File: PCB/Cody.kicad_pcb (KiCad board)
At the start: 2 copper layers, 87 x 114.5 mm, 30 parts, among them J1 Left Encoder, J12 12V Output, J13 Battery Discharge, J14 6V Input, J15 TCS34725 Color Sensor, J16 TCS34725 Color Sensor, J2 Right Encoder, J5 A1 Encoder, J6 A2 Encoder, J7 Battery Balance, J8 A3 Servo, J9 A4 Servo, U1 ESP32-DEVKITC-32D

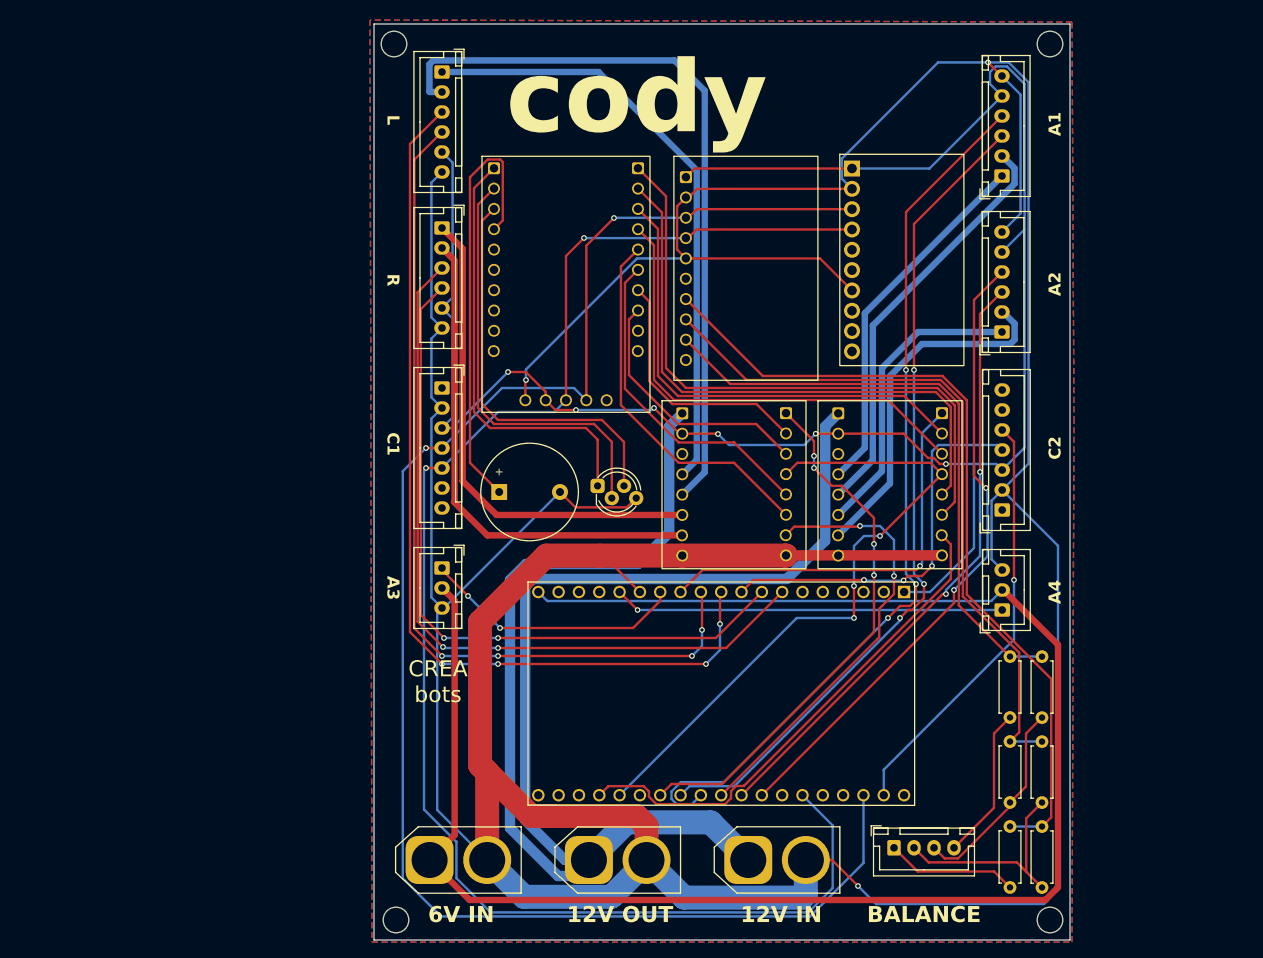
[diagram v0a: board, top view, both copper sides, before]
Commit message: 11-03-2026
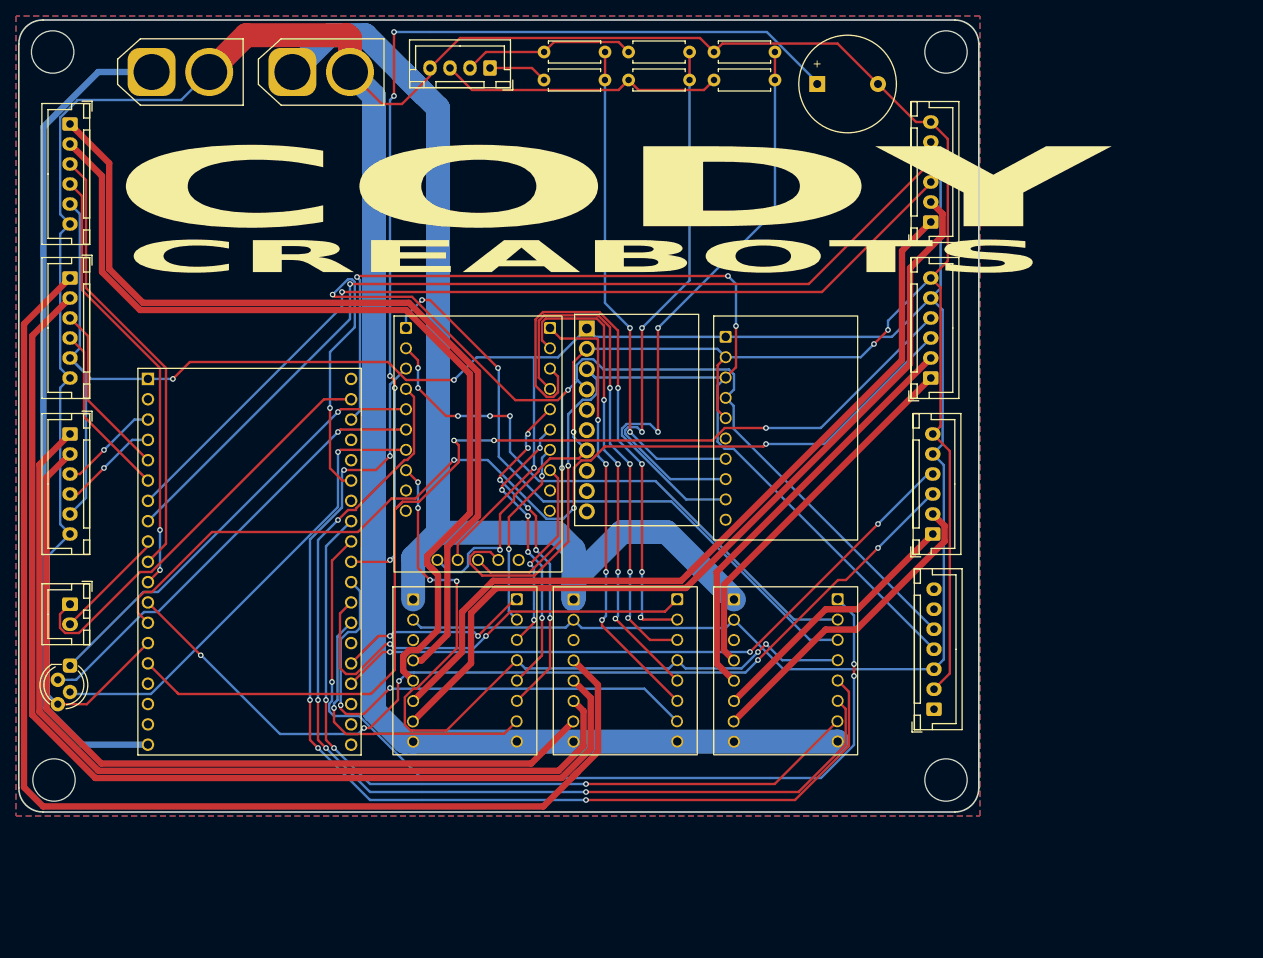
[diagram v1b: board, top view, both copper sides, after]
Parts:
- removed ? (x4): , 
- removed J12: 12V Output, Connector_AMASS:AMASS_XT60-F_1x02_P7.20mm_Vertical
- removed J16: TCS34725 Color Sensor, Connector_JST:JST_XH_B7B-XH-A_1x07_P2.50mm_Vertical
- removed J9: A4 Servo, Connector_JST:JST_XH_B3B-XH-A_1x03_P2.50mm_Vertical
- added J3: A3 Encoder, Connector_JST:JST_XH_B6B-XH-A_1x06_P2.50mm_Vertical, F.Cu at (146.6, 75.8)
- added J4: A4 Encoder, Connector_JST:JST_XH_B6B-XH-A_1x06_P2.50mm_Vertical, F.Cu at (146.8, 95.2)
- added REF**: MountingHole_5.3mm_M5, MountingHole:MountingHole_5.3mm_M5, F.Cu at (148.5, 35.0)
- added REF**: MountingHole_5.3mm_M5, MountingHole:MountingHole_5.3mm_M5, F.Cu at (36.8, 35.0)
- added REF**: MountingHole_5.3mm_M5, MountingHole:MountingHole_5.3mm_M5, F.Cu at (37.0, 126.0)
- added REF**: MountingHole_5.3mm_M5, MountingHole:MountingHole_5.3mm_M5, F.Cu at (148.5, 126.0)
- added U7: ~, Dependencies:TB6612FNG, F.Cu at (128.5, 111.3)
- J8: value A3 Servo -> Camera; footprint Connector_JST:JST_XH_B3B-XH-A_1x03_P2.50mm_Vertical -> Connector_JST:JST_XH_B2B-XH-A_1x02_P2.50mm_Vertical
- moved J5 117.2 mm to (39.0, 63.2), turned to -90 degrees
- moved J6 117.2 mm to (39.0, 82.8), turned to -90 degrees
- moved R1 116.5 mm to (98.2, 38.5), turned to 0 degrees
- moved J13 113.8 mm to (66.8, 37.5)
- moved R2 111.2 mm to (105.9, 35.0), turned to 180 degrees
- moved J7 109.8 mm to (91.5, 37.0), turned to 180 degrees
- moved R3 107.1 mm to (108.8, 35.0), turned to 0 degrees
- moved J14 104.5 mm to (49.2, 37.5)
- moved R4 91.9 mm to (116.4, 38.5), turned to 180 degrees
- moved R5 89.6 mm to (119.5, 38.5), turned to 0 degrees
- moved R6 81.1 mm to (127.1, 35.0), turned to 180 degrees
- moved J15 73.4 mm to (147.0, 117.2), turned to 90 degrees
- moved D1 69.7 mm to (39.0, 111.7), turned to -90 degrees
- moved U1 65.1 mm to (61.4, 95.6), turned to 0 degrees
- moved BZ1 64.7 mm to (132.4, 39.0)
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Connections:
- J7 pad 4: /BMS_IN_4 -> GND
- J8 pad 1: /A3 -> /CAM_TX
- J8 pad 2: +6V -> /CAM_RX
- R6 pad 2: /BMS_IN_4 -> GND
- U1 pad J2-12: /A1_PWM -> /A4_A
- U1 pad J2-13: /A3 -> /A3_A
- U1 pad J2-15: /A4 -> /A3_B
- U1 pad J2-3: unconnected-(U1-SENSOR_VP-PadJ2-3) -> /A2_A
- U1 pad J2-4: unconnected-(U1-SENSOR_VN-PadJ2-4) -> /A2_B
- U1 pad J2-5: unconnected-(U1-IO34-PadJ2-5) -> /A1_A
- U1 pad J2-6: unconnected-(U1-IO35-PadJ2-6) -> /A1_B
- U1 pad J2-9: /SCL_1 -> /CAM_RX
- U1 pad J3-10: /R_PWM -> /BUZZER
- U1 pad J3-11: /A1_B -> /A2_PWM
- U1 pad J3-12: /A1_A -> /A1_PWM
- U1 pad J3-13: /L_PWM -> /R_PWM
- U1 pad J3-15: /STNDBY -> /L_PWM
- U1 pad J3-16: /A2_PWM -> /A4_B
- U1 pad J3-2: /SDA_1 -> /CAM_TX
- U1 pad J3-8: /A2_B -> /A4_PWM
- U1 pad J3-9: /A2_A -> /A3_PWM
- U2 pad 3: (no net) -> unconnected-(U2-GND-Pad3)
- U3 pad 3: (no net) -> unconnected-(U3-GND-Pad3)
- U6 pad 1: /LED_R -> /A3_IN_1
- U6 pad 2: /LED_G -> /A3_IN_2
- U6 pad 3: /LED_B -> /A4_IN_1
- U6 pad 4: /BUZZER -> /A4_IN_2
- U6 pad 5: unconnected-(U6-P14-Pad5) -> /LED_R
- U6 pad 6: unconnected-(U6-P15-Pad6) -> /LED_G
- U6 pad 7: unconnected-(U6-P16-Pad7) -> /LED_B
- U6 pad 8: unconnected-(U6-P17-Pad8) -> /STNDBY
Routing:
- net /A4_IN_1: track 0.00 -> 135.8 mm, vias 0 -> 5
- net /A3_B: track 0.00 -> 134.2 mm, vias 0 -> 3
- net /A4_IN_2: track 0.00 -> 127.1 mm, vias 0 -> 4
- net /A3_A: track 0.00 -> 125.2 mm, vias 0 -> 3
- net /A4_A: track 0.00 -> 118.8 mm, vias 0 -> 5
- net +6V: track 216.8 -> 103.8 mm
- net /A3_PWM: track 0.00 -> 112.2 mm, vias 0 -> 3
- net /A1_OUT_1: track 45.8 -> 155.2 mm
- net /A4_PWM: track 0.00 -> 98.1 mm, vias 0 -> 3
- net /A1_B: track 111.8 -> 21.9 mm, vias 3 -> 0
- net /A1_OUT_2: track 52.1 -> 138.1 mm
- net /A4_B: track 0.00 -> 83.6 mm, vias 0 -> 3
- net /A1_A: track 103.7 -> 21.8 mm, vias 3 -> 0
- net /A3_IN_1: track 0.00 -> 80.3 mm, vias 0 -> 2
- net +3V3: track 244.6 -> 324.7 mm, vias 6 -> 3
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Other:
- board size 87 x 114.5 mm -> 120 x 99 mm
- board text added: "CODY"
- board text added: "CREABOTS"
- board text removed: "12V IN"
- board text removed: "12V OUT"
- board text removed: "6V IN"
- board text removed: "A1"
- board text removed: "A2"
- board text removed: "A3"
- board text removed: "A4"
- board text removed: "BALANCE"
- board text removed: "C1"
- board text removed: "C2"
- board text removed: "CREA bots"
- board text removed: "L"
- board text removed: "R"
- board text removed: "cody"

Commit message: 18-03-2026
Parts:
- added J10: Limit Switch 2, Connector_JST:JST_XH_B2B-XH-A_1x02_P2.50mm_Vertical, F.Cu at (100.0, 76.0)
- added J9: Limit Switch 1, Connector_JST:JST_XH_B2B-XH-A_1x02_P2.50mm_Vertical, F.Cu at (100.0, 85.2)
- added R7: R, Resistor_THT:R_Axial_DIN0207_L6.3mm_D2.5mm_P7.62mm_Horizontal, F.Cu at (121.0, 134.0)
- added SW3: SW_Push, Button_Switch_Keyboard:SW_Cherry_MX_1.00u_PCB, F.Cu at (99.4, 65.6)
- D1: value LED_RGBK -> LED; footprint LED_THT:LED_D5.0mm-4_RGB_Staggered_Pins -> LED_THT:LED_D3.0mm
- J8: footprint Connector_JST:JST_XH_B2B-XH-A_1x02_P2.50mm_Vertical -> Connector_JST:JST_XH_B4B-XH-A_1x04_P2.50mm_Vertical
- moved J14 166.7 mm to (208.5, 86.5), turned to -90 degrees
- moved J13 156.3 mm to (208.5, 103.5), turned to -90 degrees
- moved J8 148.5 mm to (175.5, 45.5), turned to 180 degrees
- moved J7 147.7 mm to (209.0, 126.5), turned to 90 degrees
- moved R2 140.4 mm to (203.4, 136.0)
- moved R1 135.5 mm to (195.8, 132.5)
- moved R3 123.8 mm to (185.2, 132.5)
- moved R4 123.8 mm to (192.8, 136.0)
- moved R5 112.1 mm to (174.8, 136.0)
- moved R6 112.1 mm to (182.4, 132.5)
- moved J6 107.2 mm to (139.5, 45.5), turned to 180 degrees
- moved J15 87.7 mm to (197.5, 45.5), turned to 180 degrees
- moved J5 82.4 mm to (119.5, 45.5), turned to 180 degrees
- moved U4 82.2 mm to (192.1, 90.3)
- moved J1 79.2 mm to (100.0, 94.5)
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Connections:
- D1 pad 1: /LED_R -> GND
- D1 pad 2: /LED_G -> Net-(D1-A)
- J1 pad 3: /L_A -> GND
- J1 pad 4: /L_B -> +3V3
- J1 pad 5: +3V3 -> /L_A
- J1 pad 6: GND -> /L_B
- J2 pad 3: /R_A -> GND
- J2 pad 4: /R_B -> +3V3
- J2 pad 5: +3V3 -> /R_A
- J2 pad 6: GND -> /R_B
- J3 pad 3: /A3_A -> GND
- J3 pad 4: /A3_B -> +3V3
- J3 pad 5: +3V3 -> /A3_A
- J3 pad 6: GND -> /A3_B
- J4 pad 3: /A4_A -> GND
- J4 pad 4: /A4_B -> +3V3
- J4 pad 5: +3V3 -> /A4_A
- J4 pad 6: GND -> /A4_B
- J5 pad 3: /A1_A -> GND
- J5 pad 4: /A1_B -> +3V3
- J5 pad 5: +3V3 -> /A1_A
- J5 pad 6: GND -> /A1_B
- J6 pad 3: /A2_A -> GND
- J6 pad 4: /A2_B -> +3V3
- J6 pad 5: +3V3 -> /A2_A
- J6 pad 6: GND -> /A2_B
- J8 pad 1: /CAM_TX -> +6V
- J8 pad 2: /CAM_RX -> GND
- U2 pad 12: /STNDBY -> +3V3
- U3 pad 12: /STNDBY -> +3V3
- U6 pad 5: /LED_R -> /LED
- U6 pad 6: /LED_G -> /LIMIT_1
- U6 pad 7: /LED_B -> /LIMIT_2
- U6 pad 8: /STNDBY -> /BUTTON
- U7 pad 12: /STNDBY -> +3V3
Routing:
- net +6V: track 103.8 -> 205.8 mm, vias 0 -> 2
- net /STNDBY: track 100.4 -> 0.00 mm, vias 6 -> 0
- net /A4_A: track 118.8 -> 20.6 mm, vias 5 -> 1
- net /CAM_RX: track 14.4 -> 107.2 mm, vias 0 -> 2
- net +3V3: track 324.7 -> 413.2 mm, vias 3 -> 4
- net /SCL: track 186.4 -> 117.7 mm, vias 4 -> 1
- net /BUTTON: track 0.00 -> 68.4 mm, vias 0 -> 1
- net +12V: track 143.1 -> 74.8 mm
- net /LED: track 0.00 -> 64.5 mm, vias 0 -> 2
- net /A4_OUT_1: track 33.5 -> 97.2 mm
- net /R_OUT_1: track 100.4 -> 160.9 mm
- net /LED_B: track 58.8 -> 0.00 mm, vias 1 -> 0
- net /LED_G: track 56.5 -> 0.00 mm, vias 1 -> 0
- net /LED_R: track 55.3 -> 0.00 mm, vias 1 -> 0
- net /SDA: track 168.1 -> 113.3 mm, vias 4 -> 1
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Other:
- board size 120 x 99 mm -> 125 x 99.9 mm
- board text added: "12V"
- board text added: "6V"
- board text added: "BALANCE"
- board text added: "CAM"
- board text added: "COLOR"
- board text added: "LEFT"
- board text added: "MILL"
- board text added: "RIGHT"
- board text added: "WHEEL"
- board text added: "X"
- board text added: "Z"
- board text added: "creabots"
- board text removed: "CREABOTS"
